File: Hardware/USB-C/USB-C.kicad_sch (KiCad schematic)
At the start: 8 parts, among them J101 USB_C_Receptacle, J102 USB_C_Receptacle

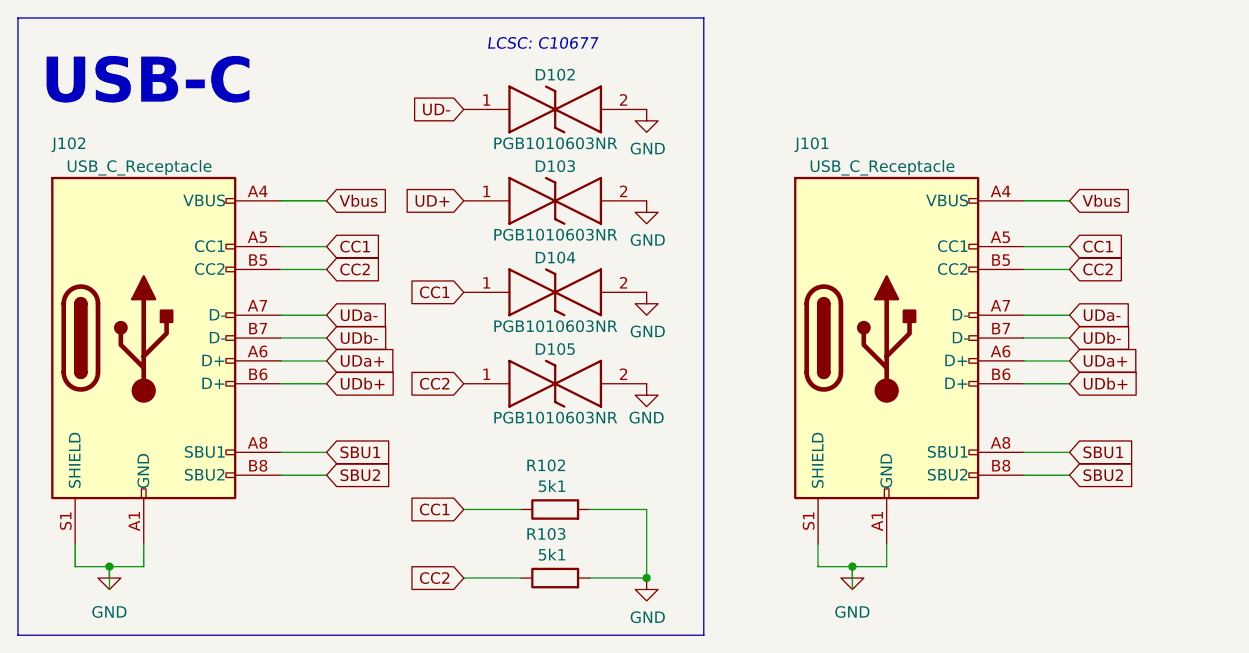
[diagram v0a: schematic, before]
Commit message: ...
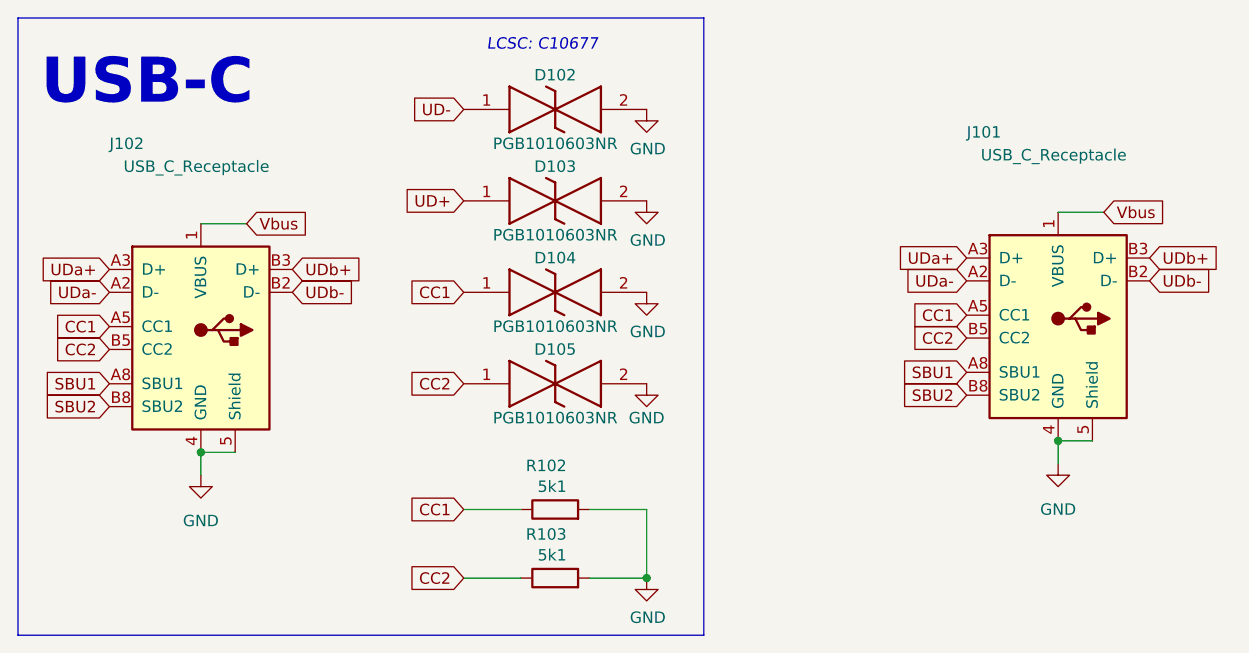
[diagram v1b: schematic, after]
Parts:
- J101, J102: footprint tinker:USB_C_Receptacle_HRO_TYPE-C-NARROW -> tinker:USB_C(sd); symbol New_Library:USB_C_Receptacle -> New_Library:USB_C(sd); LCSC C2765186 -> A-(C6389922) C-(C2765186) XT30-(C2913282)
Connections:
- net GND: now also J101.4 (GND), J101.5 (Shield), J102.4 (GND), J102.5 (Shield); no longer J101.A1 (GND), J101.A12 (GND), J101.S1 (SHIELD), J102.A1 (GND), J102.A12 (GND), J102.S1 (SHIELD)
- net UDa+: now also J101.A3 (D+), J102.A3 (D+); no longer J101.A6 (D+), J102.A6 (D+)
- net UDa-: now also J101.A2 (D-), J102.A2 (D-); no longer J101.A7 (D-), J102.A7 (D-)
- net UDb+: now also J101.B3 (D+), J102.B3 (D+); no longer J101.B6 (D+), J102.B6 (D+)
- net UDb-: now also J101.B2 (D-), J102.B2 (D-); no longer J101.B7 (D-), J102.B7 (D-)
- net Vbus: now also J101.1 (VBUS), J102.1 (VBUS); no longer J101.A4 (VBUS), J101.A9 (VBUS), J102.A4 (VBUS), J102.A9 (VBUS)
